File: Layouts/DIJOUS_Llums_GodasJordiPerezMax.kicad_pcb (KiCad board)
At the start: 2 copper layers, 84 parts, among them J1 Conn_01x05_Socket, J10 Screw_Terminal_01x02, J11 Conn_01x06, J5 Conn_01x05, J6 Conn_01x03, J7 Conn_01x02, J8 DE9_Plug, J9 Conn_01x06_Socket, Q3 Si7336ADP, Q4 Si7336ADP, Q7 Si7336ADP, Q8 Si7336ADP, U2 LM2596T-ADJ, U3 PIC18F2580-I/SO, U4 MCP2551-I-SN, U7 PCA9306D, k2 1k

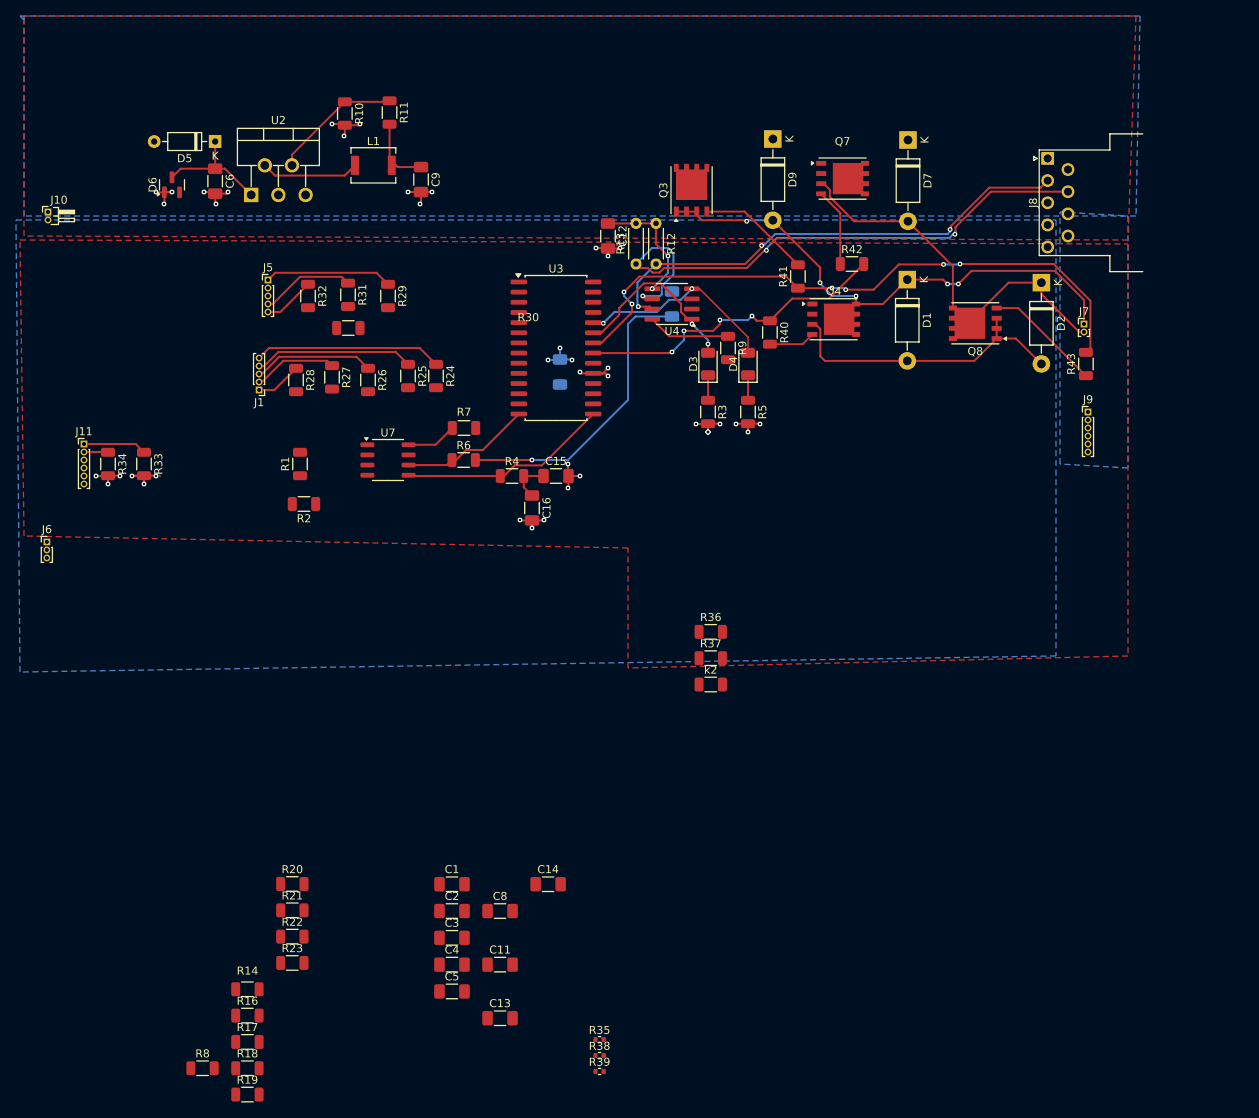
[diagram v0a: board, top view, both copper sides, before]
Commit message: Update DIJOUS_Llums_GodasJordiPerezMax.kicad_pcb
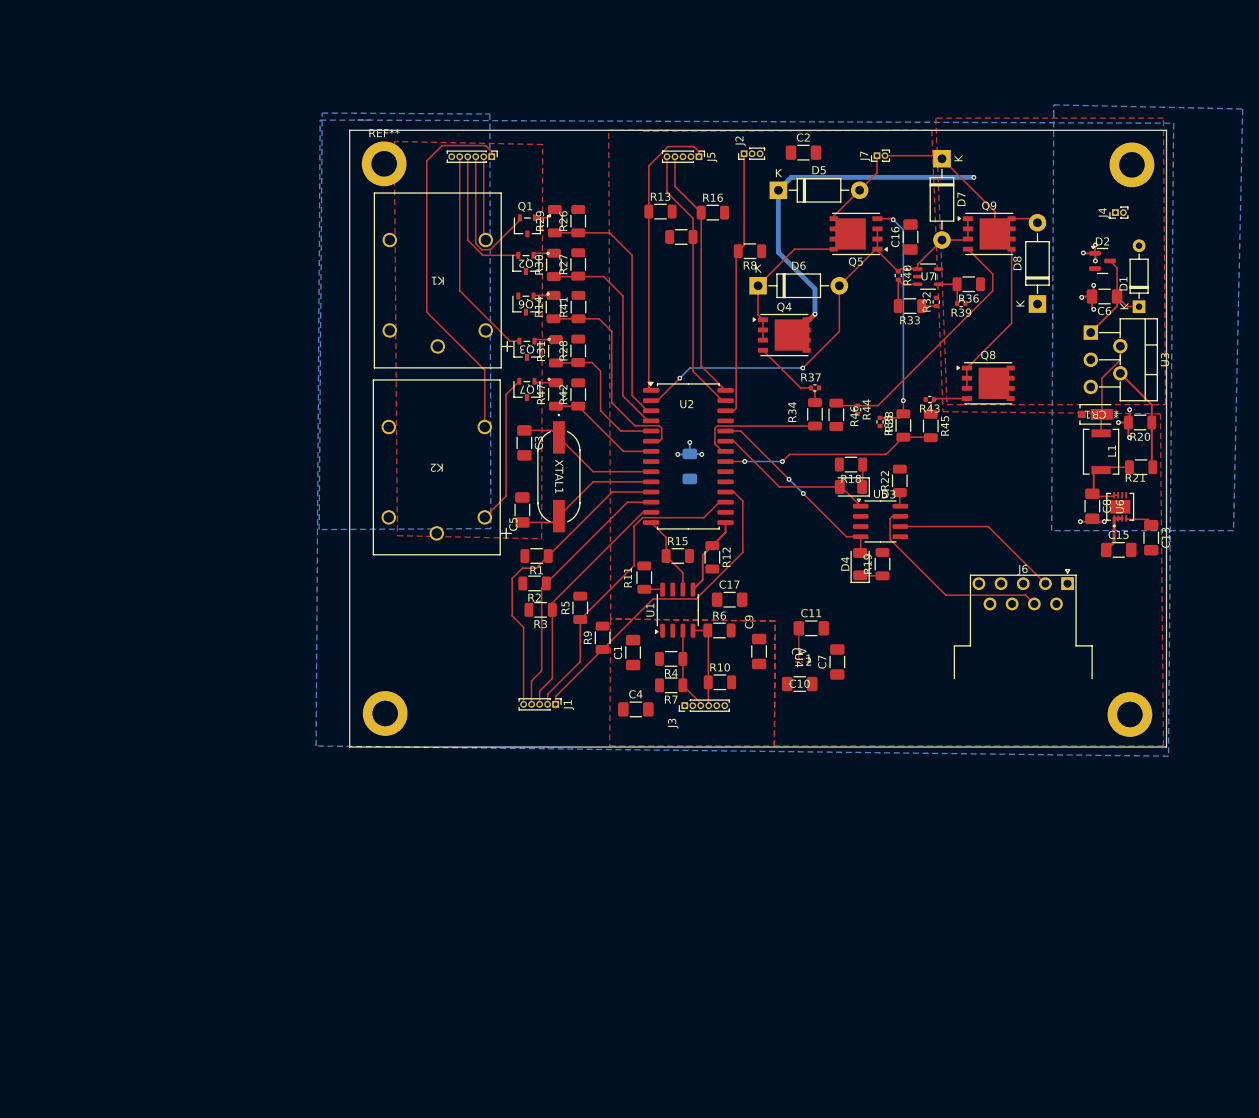
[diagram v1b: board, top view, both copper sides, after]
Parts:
- removed the C1 at (65.5, 120.5)
- removed C12: 47nF, Capacitor_SMD:C_1206_3216Metric_Pad1.33x1.80mm_HandSolder
- removed the C5 at (65.5, 133.9)
- removed the D1 at (122.4, 45.0)
- removed the D2 at (139.2, 45.3)
- removed D9: 1N5817, Diode_THT:D_DO-41_SOD81_P10.16mm_Horizontal
- removed J11: Conn_01x06, Connector_PinHeader_1.00mm:PinHeader_1x06_P1.00mm_Vertical
- removed the J8 at (140.0, 29.8)
- removed the R12 at (91.0, 37.9)
- removed R24, R25: 1k, Resistor_SMD:R_1206_3216Metric
- removed the R26 at (55.0, 57.5)
- removed the R27 at (50.5, 57.2)
- removed the R28 at (46.0, 57.5)
- removed the R29 at (57.5, 47.0)
- removed the R30 at (52.5, 51.0)
- removed the R31 at (52.5, 46.8)
- removed the R32 at (47.5, 47.0)
- removed the R33 at (27.0, 68.0)
- removed the R40 at (105.2, 51.6)
- removed the R41 at (108.7, 44.6)
- removed the R42 at (115.5, 43.0)
- added ?: , , F.Cu at (150.5, 30.6)
- added ?: , , F.Cu at (57.1, 99.2)
- added ?: , , F.Cu at (150.2, 99.3)
- added C16: 100nF, Capacitor_SMD:C_1206_3216Metric_Pad1.33x1.80mm_HandSolder, F.Cu at (122.8, 39.6)
- added C17: 100nF, Capacitor_SMD:C_1206_3216Metric_Pad1.33x1.80mm_HandSolder, F.Cu at (100.2, 85.0)
- added C4: 100nF, Capacitor_SMD:C_1206_3216Metric_Pad1.33x1.80mm_HandSolder, F.Cu at (88.5, 98.7)
- added CR1: SS3P5HM3/84A, SS3P5:CR_5HM3&slash_84A_VIS, F.Cu at (145.9, 61.8)
- added D5: 1N5817, Diode_THT:D_DO-41_SOD81_P10.16mm_Horizontal, F.Cu at (106.3, 33.8)
- added D6: 1N5817, Diode_THT:D_DO-41_SOD81_P10.16mm_Horizontal, F.Cu at (103.8, 45.7)
- added D8: 1N5817, Diode_THT:D_DO-41_SOD81_P10.16mm_Horizontal, F.Cu at (138.7, 48.0)
- added J2: Conn_01x03, Connector_PinHeader_1.00mm:PinHeader_1x03_P1.00mm_Vertical, F.Cu at (102.0, 29.2)
- added J3: Conn_01x06, Connector_PinHeader_1.00mm:PinHeader_1x06_P1.00mm_Vertical, F.Cu at (94.6, 98.2)
- added K1: G5LE-1 DC12, G5LE-1-DC12:RELAY_G5LE-1 DC5_OMR, F.Cu at (63.7, 36.8)
- added K2: G5LE-1 DC12, G5LE-1-DC12:RELAY_G5LE-1 DC5_OMR, F.Cu at (63.6, 60.2)
- added Q1: ZXTN19020DFFTA, ZXTN:ZXTN19020DFFTA_DIO, F.Cu at (74.9, 38.2)
- added Q2: ZXTN19020DFFTA, ZXTN:ZXTN19020DFFTA_DIO, F.Cu at (74.7, 42.9)
- added Q5: Si7336ADP, Package_SO:PowerPAK_SO-8_Single, F.Cu at (116.0, 39.2)
- added Q6: ZXTN19020DFFTA, ZXTN:ZXTN19020DFFTA_DIO, F.Cu at (74.7, 48.0)
- added Q9: Si7336ADP, Package_SO:PowerPAK_SO-8_Single, F.Cu at (132.7, 39.2)
- added R1: 1k, Resistor_SMD:R_1206_3216Metric, F.Cu at (76.1, 79.5)
- added R16: 1k, Resistor_SMD:R_1206_3216Metric, F.Cu at (98.1, 36.6)
- added R19: 1k, Resistor_SMD:R_1206_3216Metric, F.Cu at (119.3, 80.5)
- added R2: 1k, Resistor_SMD:R_1206_3216Metric, F.Cu at (75.8, 82.9)
- added R22: 47k, Resistor_SMD:R_1206_3216Metric, F.Cu at (121.5, 70.1)
- added R35: 1k, Resistor_SMD:R_1206_3216Metric, F.Cu at (121.9, 63.2)
- added R37: 10k, Resistor_SMD:R_0402_1005Metric, F.Cu at (110.9, 58.5)
- added R38: 10k, Resistor_SMD:R_0402_1005Metric, F.Cu at (119.0, 62.7)
- added R4: 1k, Resistor_SMD:R_1206_3216Metric, F.Cu at (92.9, 92.4)
- added R44: 10k, Resistor_SMD:R_0402_1005Metric, F.Cu at (116.2, 61.2)
- added R45: 1k, Resistor_SMD:R_1206_3216Metric, F.Cu at (125.3, 63.2)
- added R46: 1k, Resistor_SMD:R_1206_3216Metric, F.Cu at (113.5, 61.8)
- added R47: 100, Resistor_SMD:R_1206_3216Metric, F.Cu at (78.5, 59.3)
- added R6: 1k, Resistor_SMD:R_1206_3216Metric, F.Cu at (98.9, 88.8)
- added R8: 220, Resistor_SMD:R_1206_3216Metric, F.Cu at (102.7, 41.4)
- added REF**: MountingHole_3.2mm_M3_DIN965_Pad, MountingHole:MountingHole_3.2mm_M3_DIN965_Pad, F.Cu at (57.0, 30.5)
- added U5: MCP2551-I-SN, Package_SO:SOIC-8_3.9x4.9mm_P1.27mm, F.Cu at (119.1, 75.2)
- added U6: ADM7172ACPZ-5.0-R7, ADM7172ACPZ-5.0-R7:CP-8-21_ADI, F.Cu at (149.0, 73.4)
- added U7: LT6202CS5, LT6202CS5:S_5_ADI, F.Cu at (125.0, 44.6)
- added XTAL1: XT9M20ANA8M, XT9M20HRR8M:XTAL_ANA8M_VIS, F.Cu at (78.9, 69.6)
- C7: moved to F.Cu
- J4: renamed from J10; footprint Connector_PinHeader_1.00mm:PinHeader_1x02_P1.00mm_Horizontal -> Connector_PinHeader_1.00mm:PinHeader_1x02_P1.00mm_Vertical
- J6: value Conn_01x03 -> DE9_Plug; footprint Connector_PinHeader_1.00mm:PinHeader_1x03_P1.00mm_Vertical -> Connector_Dsub:DSUB-9_Female_Horizontal_P2.77x2.54mm_EdgePinOffset9.40mm
- Q3, Q7: value Si7336ADP -> ZXTN19020DFFTA; footprint Package_SO:PowerPAK_SO-8_Single -> ZXTN:ZXTN19020DFFTA_DIO
- R13: value 60 -> 1k; footprint Resistor_THT:R_Axial_DIN0204_L3.6mm_D1.6mm_P5.08mm_Horizontal -> Resistor_SMD:R_1206_3216Metric
- R14: value 220 -> 100
- R17, R18: value 100 -> 1k
- R43: value 1k -> 10k; footprint Resistor_SMD:R_1206_3216Metric -> Resistor_SMD:R_0402_1005Metric
- R9: value 47k -> 1k
- U4: value MCP2551-I-SN -> ADP7112ACBZ-3.3-R7; footprint Package_SO:SOIC-8_3.9x4.9mm_P1.27mm -> ADP7112ACBZ-3.3-R7:CB-6-15_ADI-M
- moved J4 133.4 mm to (148.4, 36.6), turned to 90 degrees
- moved J6 127.7 mm to (142.4, 83.0)
- moved D1 117.3 mm to (151.4, 48.3), turned to 90 degrees
- moved D2 116.7 mm to (146.8, 42.6), turned to 0 degrees
- moved R17 114.3 mm to (94.2, 39.6), turned to 180 degrees
- moved C6 112.1 mm to (147.1, 47.1), turned to 180 degrees
- moved R26 107.6 mm to (81.3, 37.6), turned to 90 degrees
- moved R41 106.8 mm to (81.3, 48.4), turned to 90 degrees
- moved R18 106.7 mm to (115.4, 68.1), turned to 180 degrees
- moved R20 106.6 mm to (151.5, 62.8), turned to 180 degrees
- moved U3 106.3 mm to (145.3, 51.6), turned to -90 degrees
- moved R40 106.3 mm to (121.3, 44.5), turned to -90 degrees
- moved R39 104.3 mm to (129.2, 47.9), turned to 180 degrees
- moved R21 103.9 mm to (151.6, 68.4), turned to 180 degrees
- moved R32 101.4 mm to (126.0, 47.8), turned to 90 degrees
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- renumbered C3 to C1, C8 to C10, C13 to C11, C14 to C13, C17 to C14, C16 to C15, C15 to C2, C2 to C3, C4 to C5, C9 to C8, C11 to C9, D5 to D1, D6 to D2, J9 to J8, R2 to R10, R7 to R11, R4 to R12, R6 to R15, R10 to R20, R11 to R21, R16 to R26, R21 to R27, R8 to R28, R23 to R29, R22 to R30, R20 to R31, R35 to R32, R36 to R33, k2 to R36, R38 to R39, R39 to R40, R19 to R41, R37 to R42, R1 to R7, U7 to U1, U3 to U2, U2 to U3
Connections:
- net Net-(Q8-G) renamed /BJTbase12
- net SCL renamed SCl
- net SCL_O+ renamed SCL_O
- net SDA_O- renamed SDA_O
- C1 pad 2: VREF1 -> +3.3V
- C10 pad 1: VDD-trans -> +5V
- C11 pad 1: Net-(U5-SS) -> Net-(U4-SS)
- C14 pad 1: +Vcc -> +5V
- C15 pad 1: VDD-trans -> +5V
- C2 pad 1: VDD-trans -> +5V
- C7 pad 1: VDD-trans -> +5V
- C9 pad 1: VREF1 -> +3.3V
- D3 pad 1: Net-(D3-K) -> /LEDTX
- D3 pad 2: CAN- -> CANTX
- D4 pad 1: Net-(D4-K) -> /LEDRX
- D4 pad 2: CAN+ -> CANRX
- D7 pad 1: +12V -> Motor_o2
- D7 pad 2: Motor_o2 -> Shutin
- J4 pad 2: /fuse_node -> +12V
- J5 pad 2: +Vcc -> +5V
- J6 pad 1: RB5 -> unconnected-(J6-Pad1)
- J6 pad 2: GND -> CANL_O
- J6 pad 3: GND -> unconnected-(J6-Pad3)
- Q3 pad 1: Motor_o1 -> Net-(Q3-Pad1)
- Q3 pad 2: Motor_o1 -> Brushless
- Q3 pad 3: Motor_o1 -> +12V
- Q4 pad 1: Shunt_in -> Motor_o1
- Q4 pad 2: Shunt_in -> Motor_o1
- Q4 pad 3: Shunt_in -> Motor_o1
- Q4 pad 4: Net-(Q4-G) -> /BJTbase11
- Q4 pad 5: Motor_o1 -> +12V
- Q7 pad 1: Motor_o2 -> Net-(Q7-Pad1)
- Q7 pad 2: Motor_o2 -> Net-(K2-Pad2)
- Q7 pad 3: Motor_o2 -> +12V
- Q8 pad 1: Shunt_in -> Motor_o2
- Q8 pad 2: Shunt_in -> Motor_o2
- Q8 pad 3: Shunt_in -> Motor_o2
- Q8 pad 5: Motor_o2 -> +12V
- R10 pad 2: VREF1 -> +3.3V
- R11 pad 1: +12V -> +5V
- R12 pad 2: VDD-trans -> +5V
- R13 pad 1: CANO- -> MCLR
- R13 pad 2: Vref -> GND
- R14 pad 1: VDD-trans -> RA4
- R14 pad 2: RB5 -> Net-(Q6-Pad1)
- R15 pad 2: VDD-trans -> +5V
- R17 pad 1: RB5 -> PGC
- R17 pad 2: Net-(Q2-Pad1) (its old number) -> GND
- R18 pad 1: RB5 -> /LEDTX
- R18 pad 2: GNDPWR -> GND
- R26 pad 2: GNDPWR -> GND
- R27 pad 2: GNDPWR -> GND
- R28 pad 2: GNDPWR -> GND
- R3 pad 1: Net-(D3-K) -> RC2
- R31 pad 2: Net-(Q9-Pad1) -> Net-(Q3-Pad1)
- R32 pad 2: GNDPWR -> GND
- R34 pad 1: SDA -> Motor_in1
- R34 pad 2: GND -> /BJTbase11
- R36 pad 1: GNDPWR -> GND
- R39 pad 1: GNDPWR -> GND
- R41 pad 2: GNDPWR -> GND
- R42 pad 2: GNDPWR -> GND
- R43 pad 2: Motor_in1 -> GND
- R5 pad 1: Net-(D4-K) -> RC6
- R7 pad 2: VREF1 -> +3.3V
- R9 pad 1: Net-(U4-Rs) -> RC7
- U1 pad 2: VREF1 -> +3.3V
- U1 pad 7: VREF1 -> +5V
- U2 pad 20: +Vcc -> +5V
- U2 pad 23: CAN- -> CANTX
- U2 pad 24: CAN+ -> CANRX
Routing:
- net CANO-: track 74.5 -> 0.00 mm, vias 3 -> 0
- net CANO+: track 63.0 -> 0.00 mm, vias 3 -> 0
- net Motor_in1: track 79.1 -> 16.3 mm, vias 6 -> 0
- net Shutin: track 0.00 -> 59.1 mm, vias 0 -> 2
- net +12V: track 0.00 -> 50.5 mm, vias 0 -> 2
- net Low Beam: track 0.00 -> 46.7 mm
- net VDD-trans: track 42.9 -> 0.00 mm, vias 1 -> 0
- net Shunt_in: track 37.5 -> 0.00 mm
- net Motor_o1: track 64.8 -> 28.5 mm, vias 5 -> 0
- net RC7: track 5.74 -> 40.9 mm
- net GND: track 34.6 -> 0.00 mm, vias 26 -> 0
- net RB5: track 0.00 -> 33.7 mm
- net /BJTbase22: track 0.00 -> 32.1 mm
- net RA1: track 0.00 -> 31.5 mm
- net /BJTbase21: track 0.00 -> 29.9 mm, vias 0 -> 2
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- added copper zone on F.Cu, net +3.3V
- added copper zone on F.Cu, net +5V
- removed copper zone on F.Cu, net +Vcc
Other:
- board outline added: 102.1 x 77.1 mm
